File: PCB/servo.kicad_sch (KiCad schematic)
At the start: 10 parts, among them J1 Conn_ARM_SWD_TagConnect_TC203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, U1 ATSAMD21E17D-M, U2 TMC6300-LA-T, U3 MA730, U4 LDK130PU33R_DFN6

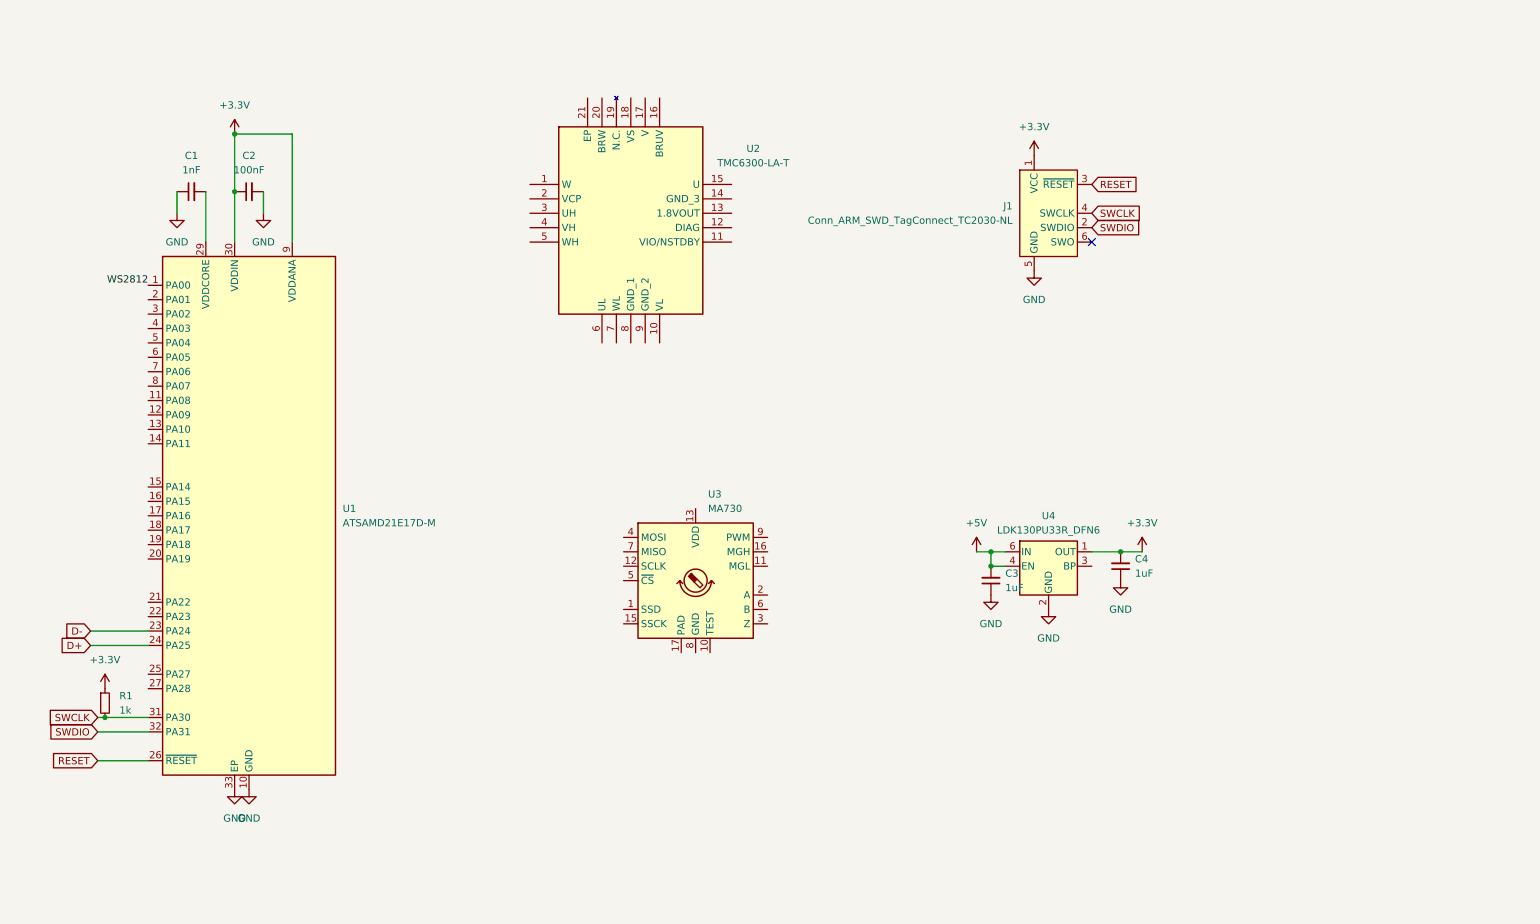
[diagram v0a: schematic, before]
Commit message: initial schematic
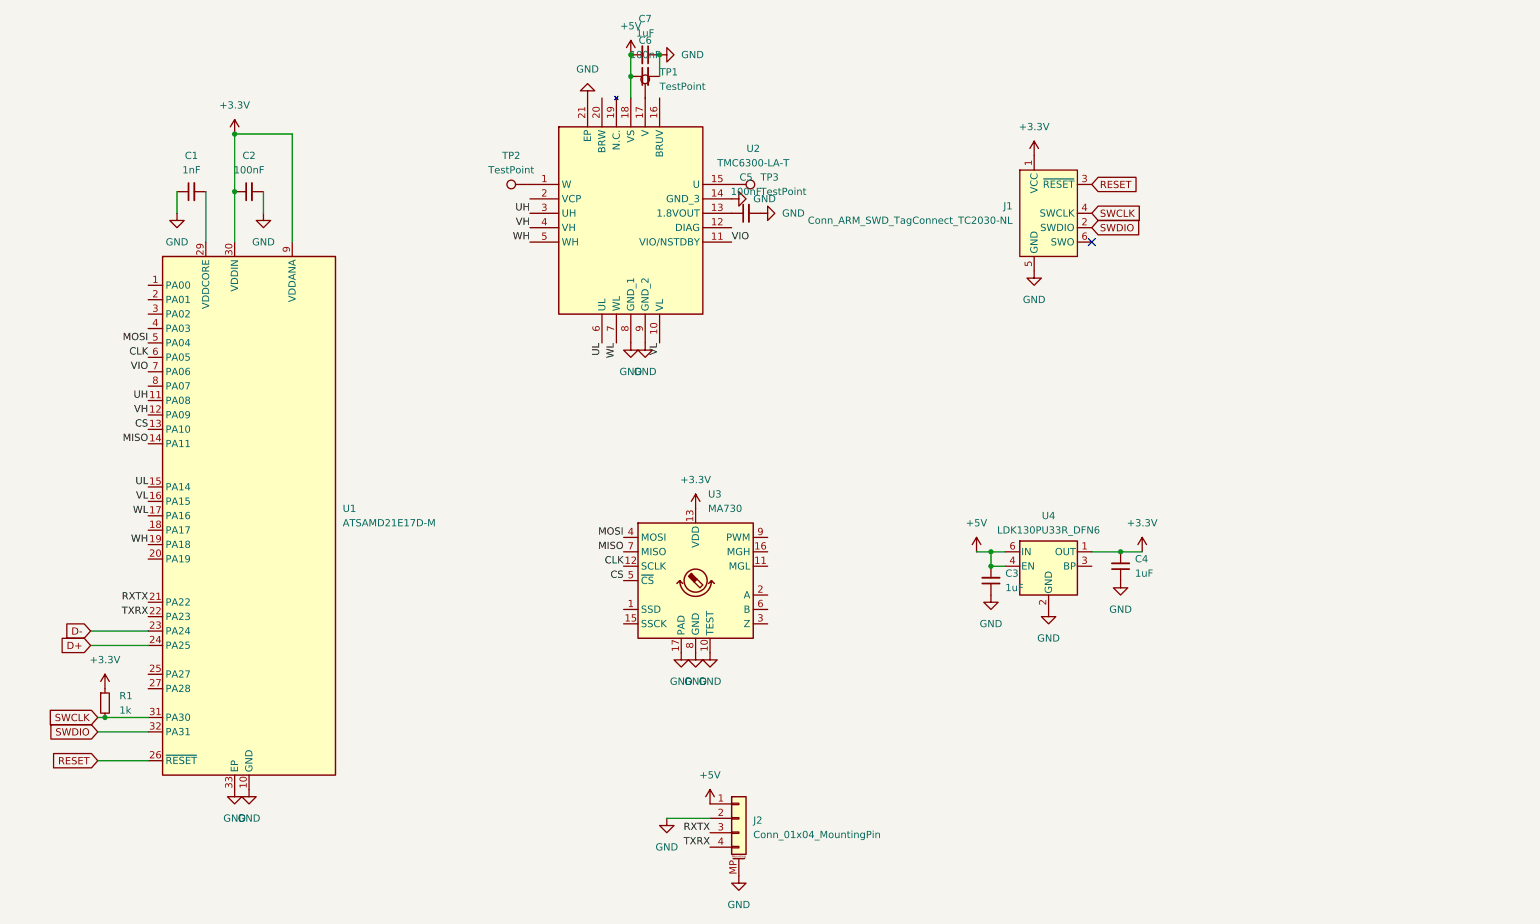
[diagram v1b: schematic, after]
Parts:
- added C5, C6: 100nF, Capacitor_SMD:C_0402_1005Metric, symbol Device:C_Small
- added C7: 1uF, Capacitor_SMD:C_0402_1005Metric, symbol Device:C_Small
- added J2: Conn_01x04_MountingPin, Connector_Molex:Molex_Pico-EZmate_78171-0004_1x04-1MP_P1.20mm_Vertical, symbol Connector_Generic_MountingPin:Conn_01x04_MountingPin
- added TP1, TP2, TP3: TestPoint, TestPoint:TestPoint_Pad_D1.5mm, symbol Connector:TestPoint
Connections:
- net +3.3V: now also U3.13 (VDD)
- net +5V: now also U2.18 (VS), C6.1, C7.2, J2.1 (Pin_1)
- net GND: now also U2.14 (GND_3), U2.21 (EP), U2.8 (GND_1), U2.9 (GND_2), U3.10 (TEST), U3.17 (PAD), U3.8 (GND), C5.2, C6.2, C7.1, J2.2 (Pin_2), J2.MP (MountPin)
- net CLK: now reaches U3.12 (SCLK)
- net CLK: now also U1.6 (PA05)
- net MOSI: now reaches U3.4 (MOSI)
- net MOSI: now also U1.5 (PA04)
- net CS: now reaches U3.5 (~{CS})
- net CS: now also U1.13 (PA10)
- net MISO: now reaches U3.7 (MISO)
- net MISO: now also U1.14 (PA11)
- net at U2.1 (W): now also TP2.1
- net VL: now reaches U2.10 (VL)
- net VL: now also U1.16 (PA15)
- net VIO: now reaches U2.11 (VIO/NSTDBY)
- net VIO: now also U1.7 (PA06)
- net at U2.13 (1.8VOUT): now also C5.1
- net at U2.15 (U): now also TP3.1
- net at U2.17 (V): now also TP1.1
- net UH: now reaches U2.3 (UH)
- net UH: now also U1.11 (PA08)
- net VH: now reaches U2.4 (VH)
- net VH: now also U1.12 (PA09)
- net WH: now reaches U2.5 (WH)
- net WH: now also U1.19 (PA18)
- net UL: now reaches U2.6 (UL)
- net UL: now also U1.15 (PA14)
- net WL: now reaches U2.7 (WL)
- net WL: now also U1.17 (PA16)
- net RXTX: now reaches U1.21 (PA22)
- net RXTX: now also J2.3 (Pin_3)
- net TXRX: now reaches U1.22 (PA23)
- net TXRX: now also J2.4 (Pin_4)
- net WS2812: no longer names the net of U1.1 (PA00)

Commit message: Commit currrent work
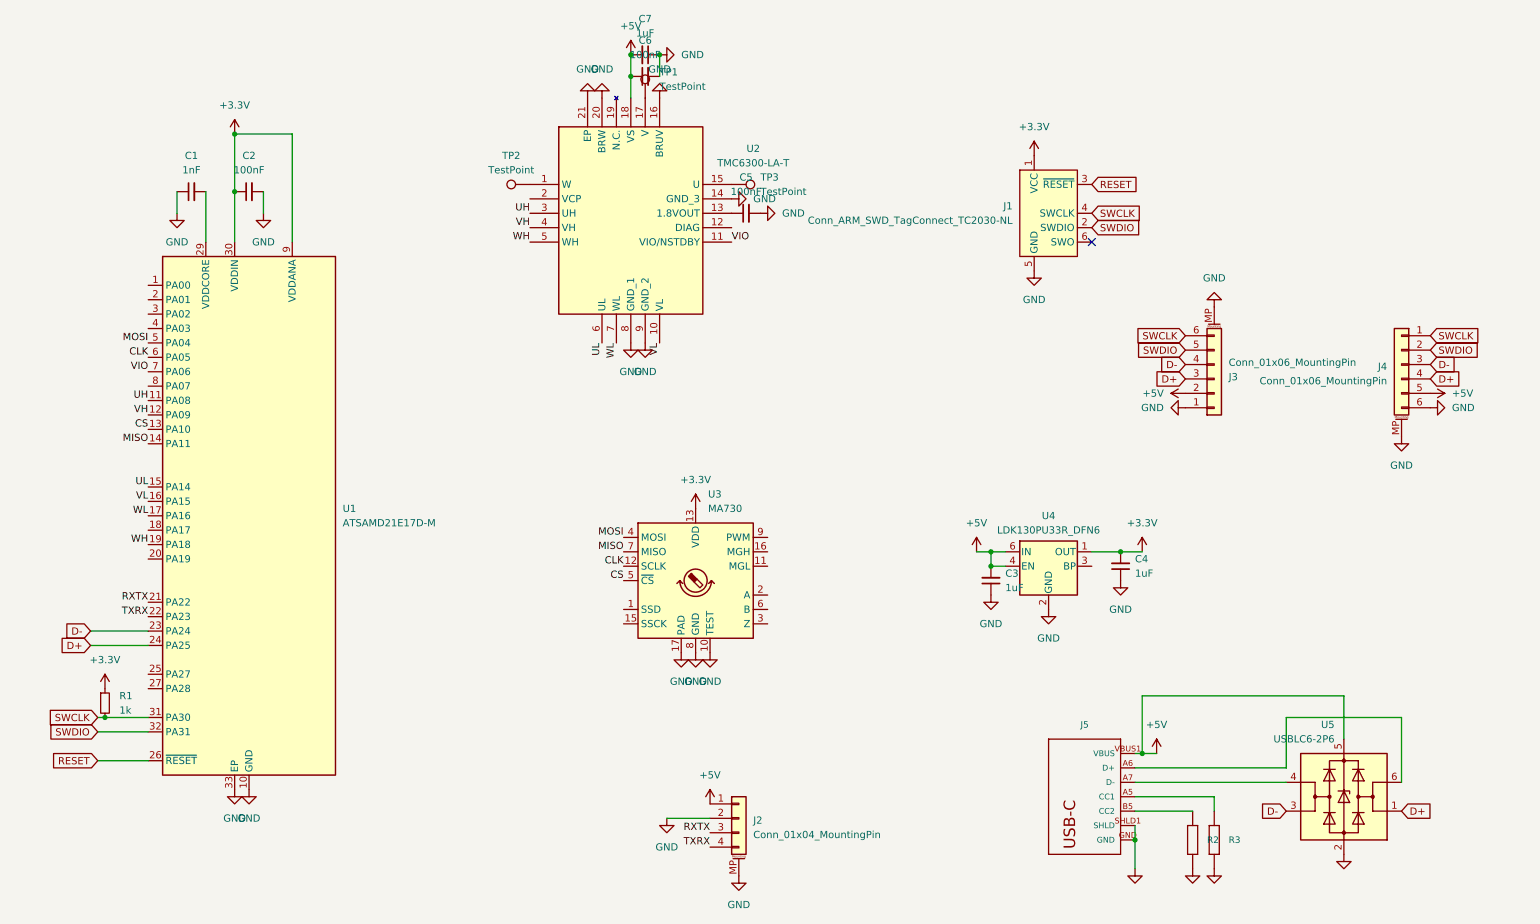
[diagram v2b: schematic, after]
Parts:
- added J3, J4: Conn_01x06_MountingPin, Connector_JST:JST_SH_SM06B-SRSS-TB_1x06-1MP_P1.00mm_Horizontal, symbol Connector_Generic_MountingPin:Conn_01x06_MountingPin
- added J5: XKB-USB-C16PIN, common:XKB-USB-C-16P, symbol ergo-pw:XKB-USB-C16PIN
- added R2, R3: 5.1k, common:R_0402_1005Metric, symbol ergo-pw:R-EU_R0603
- added U5: USBLC6-2P6, common:SOT-666, symbol ergo-pw:USBLC6-2SC6
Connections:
- net +5V: now also J3.2 (Pin_2), J4.5 (Pin_5), J5.VBUS1 (VBUS), J5.VBUS2 (VBUS), U5.5 (VBUS)
- net D+: now also J3.3 (Pin_3), J4.4 (Pin_4), U5.1 (I/O1)
- net D-: now also J3.4 (Pin_4), J4.3 (Pin_3), U5.3 (I/O2)
- net GND: now also U2.16 (BRUV), U2.20 (BRW), J3.1 (Pin_1), J3.MP (MountPin), J4.6 (Pin_6), J4.MP (MountPin), J5.GND, J5.GND2 (GND), J5.SHLD1 (SHLD), R2.1, R3.1, U5.2 (GND)
- net SWCLK: now also J3.6 (Pin_6), J4.1 (Pin_1)
- net SWDIO: now also J3.5 (Pin_5), J4.2 (Pin_2)
- new net: J5.B5 (CC2), R2.2
- new net: J5.A7 (D-), J5.B7 (D-), U5.4 (I/O2)
- new net: J5.A6 (D+), J5.B6 (D+), U5.6 (I/O1)
- new net: J5.A5 (CC1), R3.2

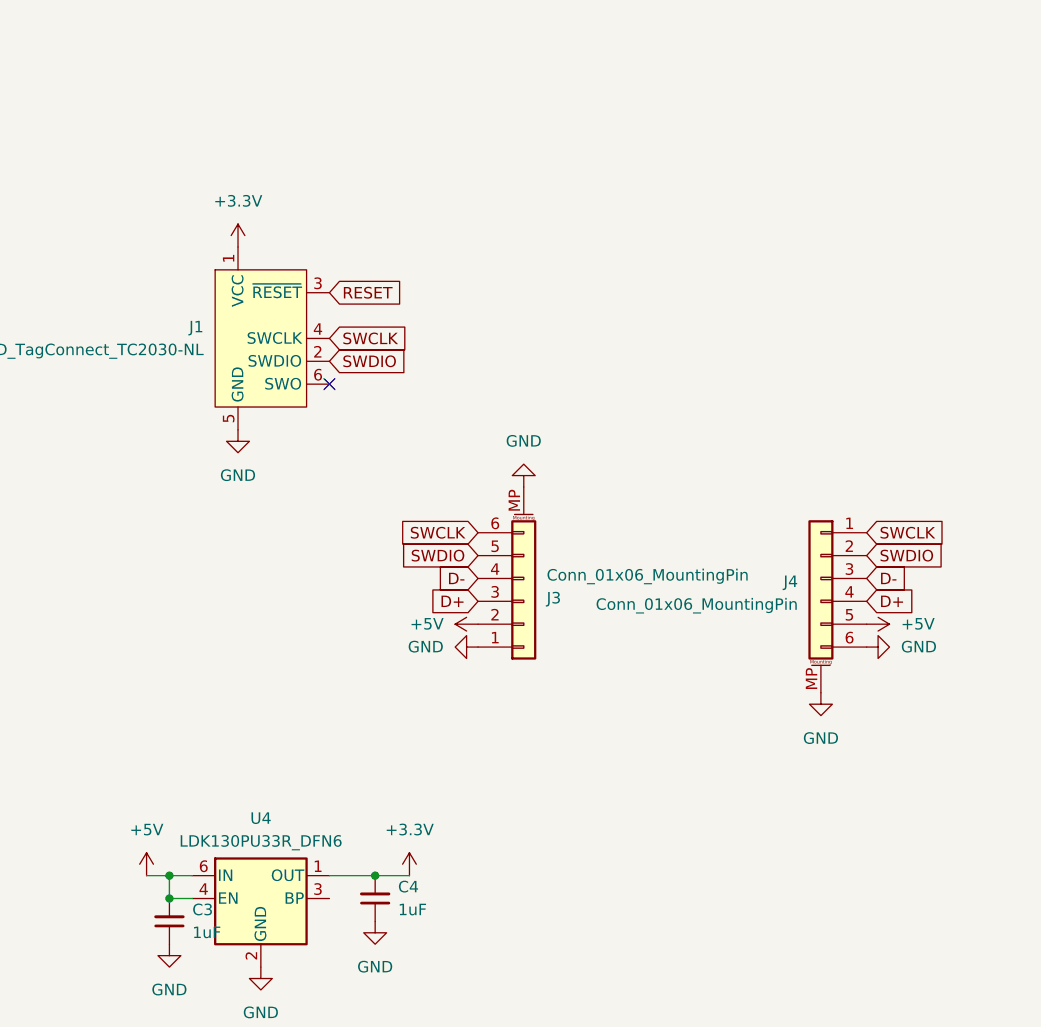
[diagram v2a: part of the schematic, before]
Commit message: Complete PCB
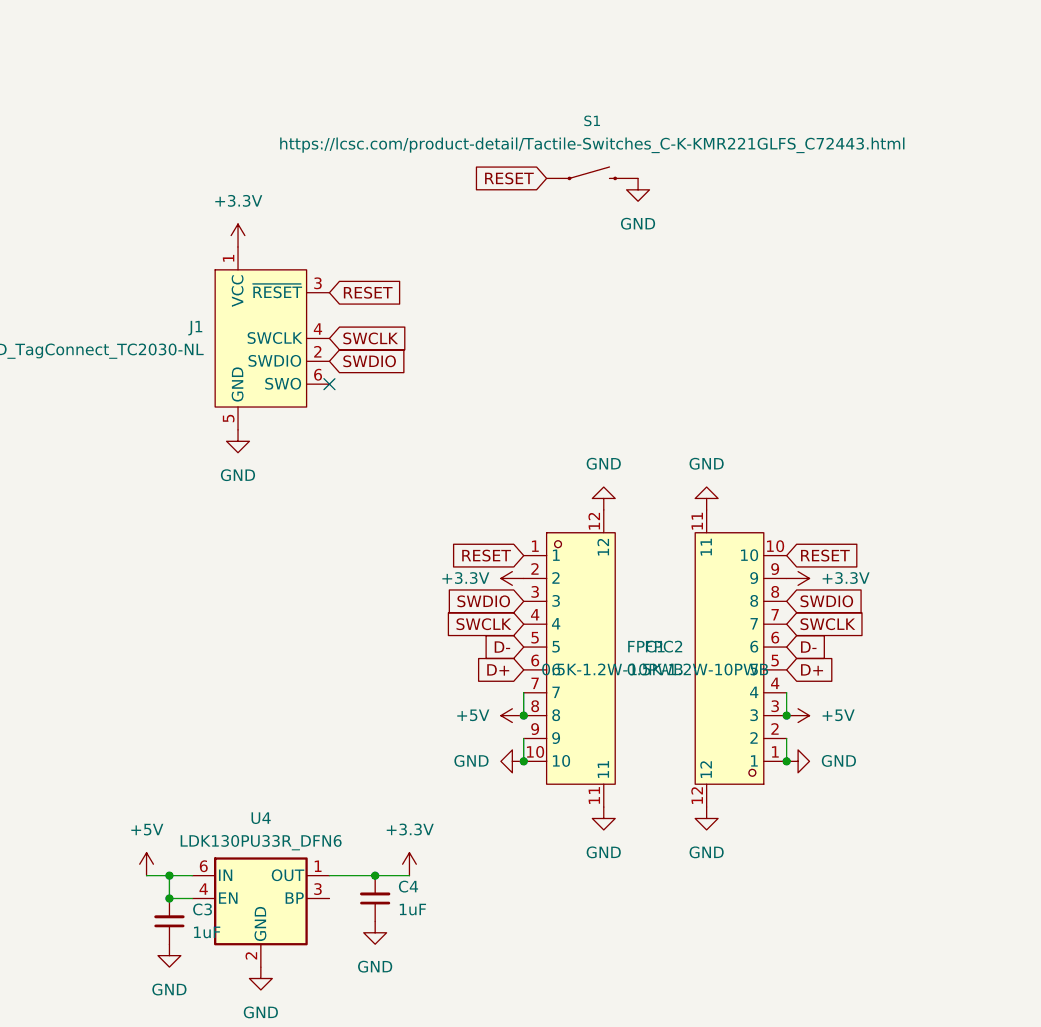
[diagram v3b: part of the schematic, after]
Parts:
- removed J3, J4: Conn_01x06_MountingPin, Connector_JST:JST_SH_SM06B-SRSS-TB_1x06-1MP_P1.00mm_Horizontal, symbol Connector_Generic_MountingPin:Conn_01x06_MountingPin
- added FPC1, FPC2: 0.5K-1.2W-10PWB, common:CONN-SMD_10P-P0.50_0.5K-1.2W-10PWB, symbol common:0.5K-1.2W-10PWB
- added S1: MOMENTARY-SWITCH-SPST-SMD-4.6X2.8MM, common:TACTILE_SWITCH_SMD_4.6X2.8MM, symbol common:MOMENTARY-SWITCH-SPST-SMD-4.6X2.8MM
- C1: LCSC Part (none) -> C129637
- C2, C3, C4, C5, C6, C7: LCSC Part (none) -> C2169363
- J2: LCSC Part (none) -> C2840019
- R1: LCSC Part (none) -> C2906899
- U1: LCSC Part (none) -> C614245
- U4: LCSC Part (none) -> C5267896
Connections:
- net +3.3V: now also FPC1.2, FPC2.9
- net +5V: now also FPC1.7, FPC1.8, FPC2.3, FPC2.4
- net D+: now also FPC1.6, FPC2.5
- net D-: now also FPC1.5, FPC2.6
- net GND: now also FPC1.10, FPC1.11, FPC1.12, FPC1.9, FPC2.1, FPC2.11, FPC2.12, FPC2.2, S1.3 (2), S1.4 (2)
- net RESET: now also FPC1.1, FPC2.10, S1.1, S1.2 (1)
- net SWCLK: now also FPC1.4, FPC2.7
- net SWDIO: now also FPC1.3, FPC2.8

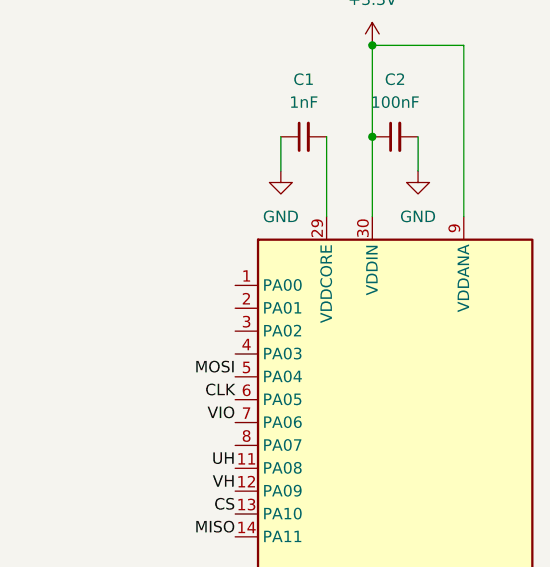
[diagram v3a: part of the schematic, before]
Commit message: Minor revisions
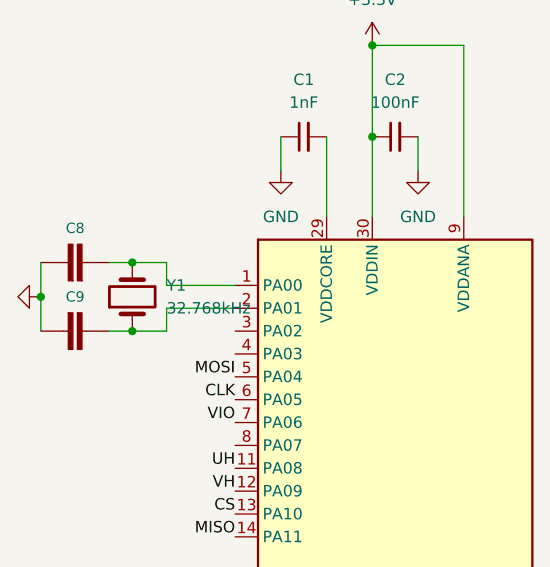
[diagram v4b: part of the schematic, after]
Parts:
- added C8, C9: 12pF, common:C_0402_1005Metric, symbol ergo-pw:C-EUC0603
- added Y1: 32.768kHz, common:Crystal_SMD_2012-2Pin_2.0x1.2mm, symbol ergo-pw:Crystal
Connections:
- net GND: now also C8.1, C9.2
- net at U1.1 (PA00): now also C8.2, Y1.2
- net at U1.2 (PA01): now also C9.1, Y1.1
